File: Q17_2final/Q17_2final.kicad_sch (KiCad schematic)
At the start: 91 parts, among them J1 Input, J2 Screw_Terminal_01x02, J3 Screw_Terminal_01x03, Q1 IRF610, Q10 2SA970, Q11 BS250, Q12 2SC2240 / AC181, Q13 IRF610, Q14 IRF9610, Q15 FQA46N15, Q16 FQA36P15, Q17 FQA46N15, Q18 FQA36P15, Q2 2SA970, Q3 2SC2240, Q4 IRF9610, Q5 FQP3P20, Q6 FQP3N30, Q7 2SC2240, Q8 2N7000, Q9 BS250, U1 OPA1641

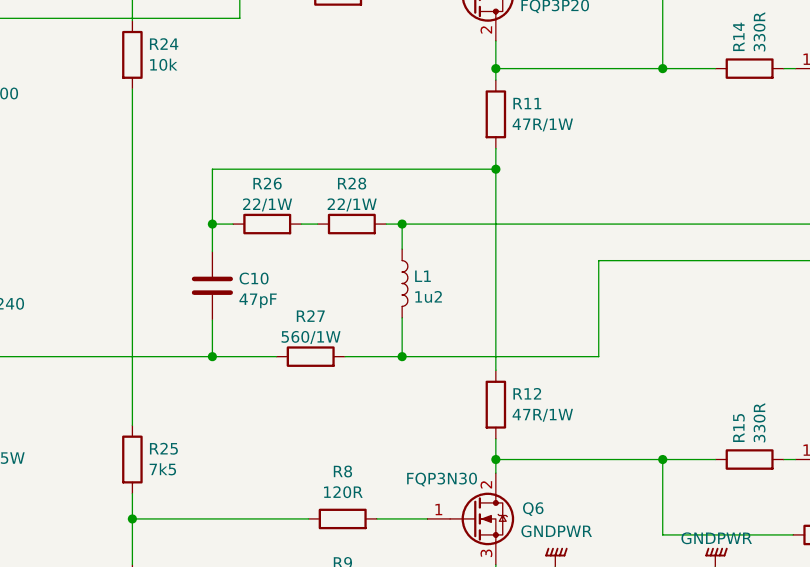
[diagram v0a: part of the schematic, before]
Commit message: Add files via upload
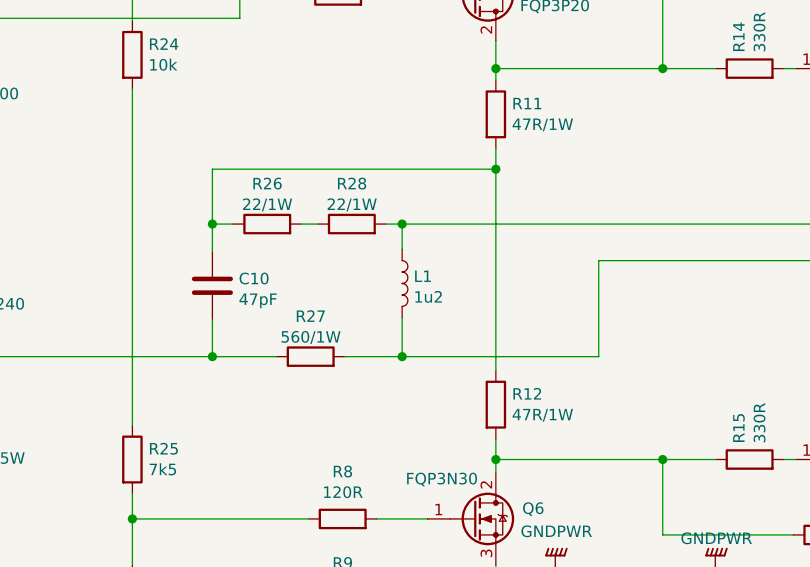
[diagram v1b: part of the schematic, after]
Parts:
- C11, C12, C18, C19, C26, C27, C4, C5, C8, C9: Spice_Model 100n -> (none); Spice_Netlist_Enabled Y -> (none); Spice_Primitive C -> (none)
